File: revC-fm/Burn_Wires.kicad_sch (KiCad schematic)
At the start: 14 parts, among them Q19 MMBT2222AWT3G, Q20 DMN100-7-F, Q21 DMN100-7-F, Q22 IRF7404TRPBF, Q23 IRF7404TRPBF, U23 PE014006

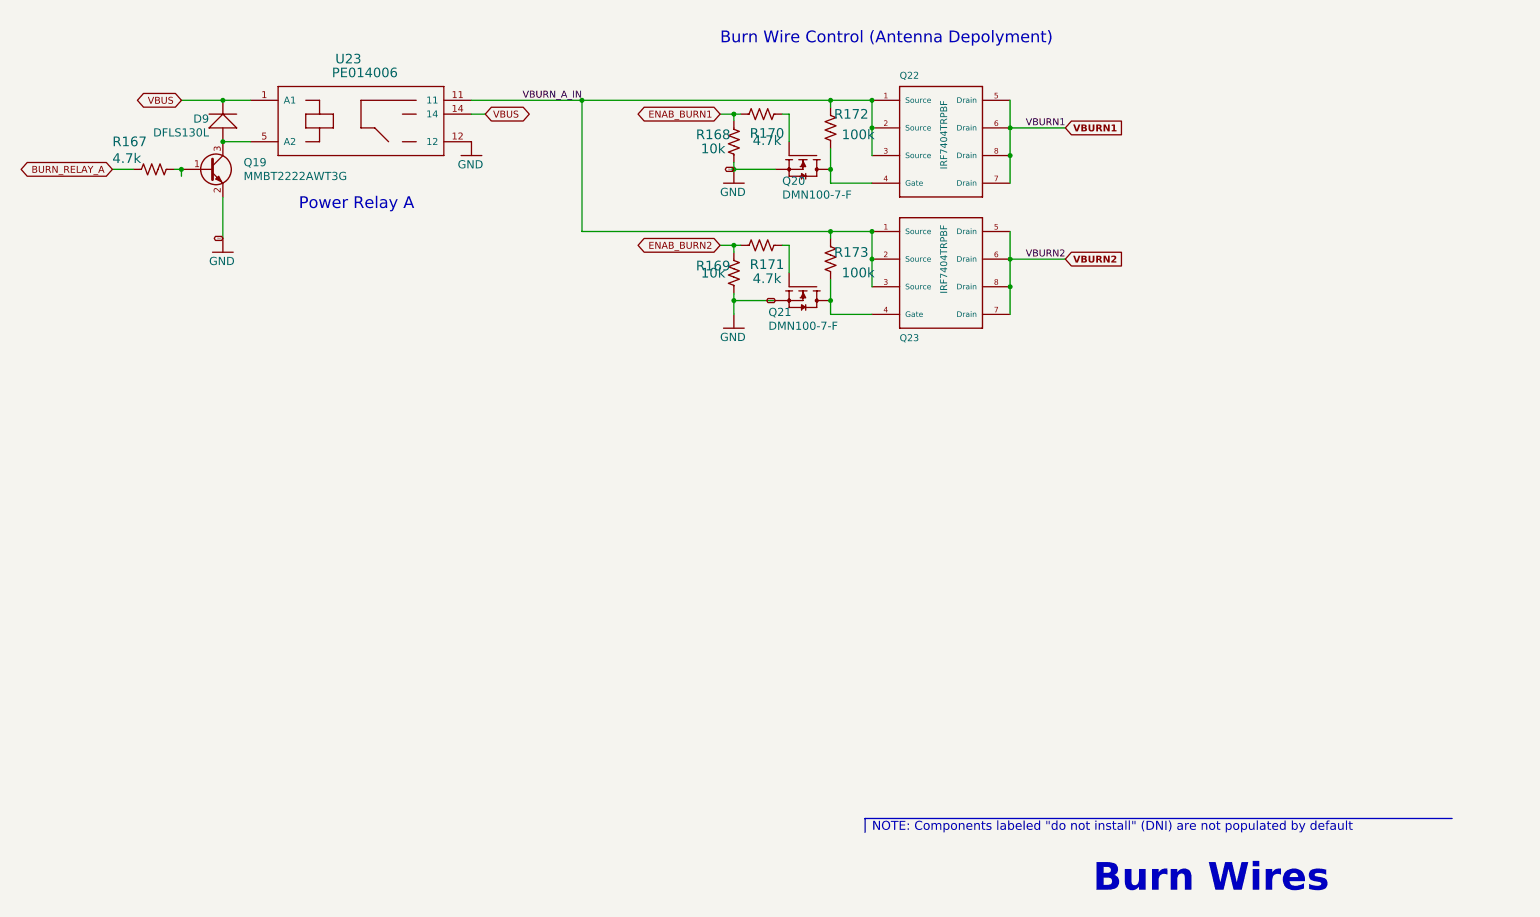
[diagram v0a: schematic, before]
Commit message: working revC
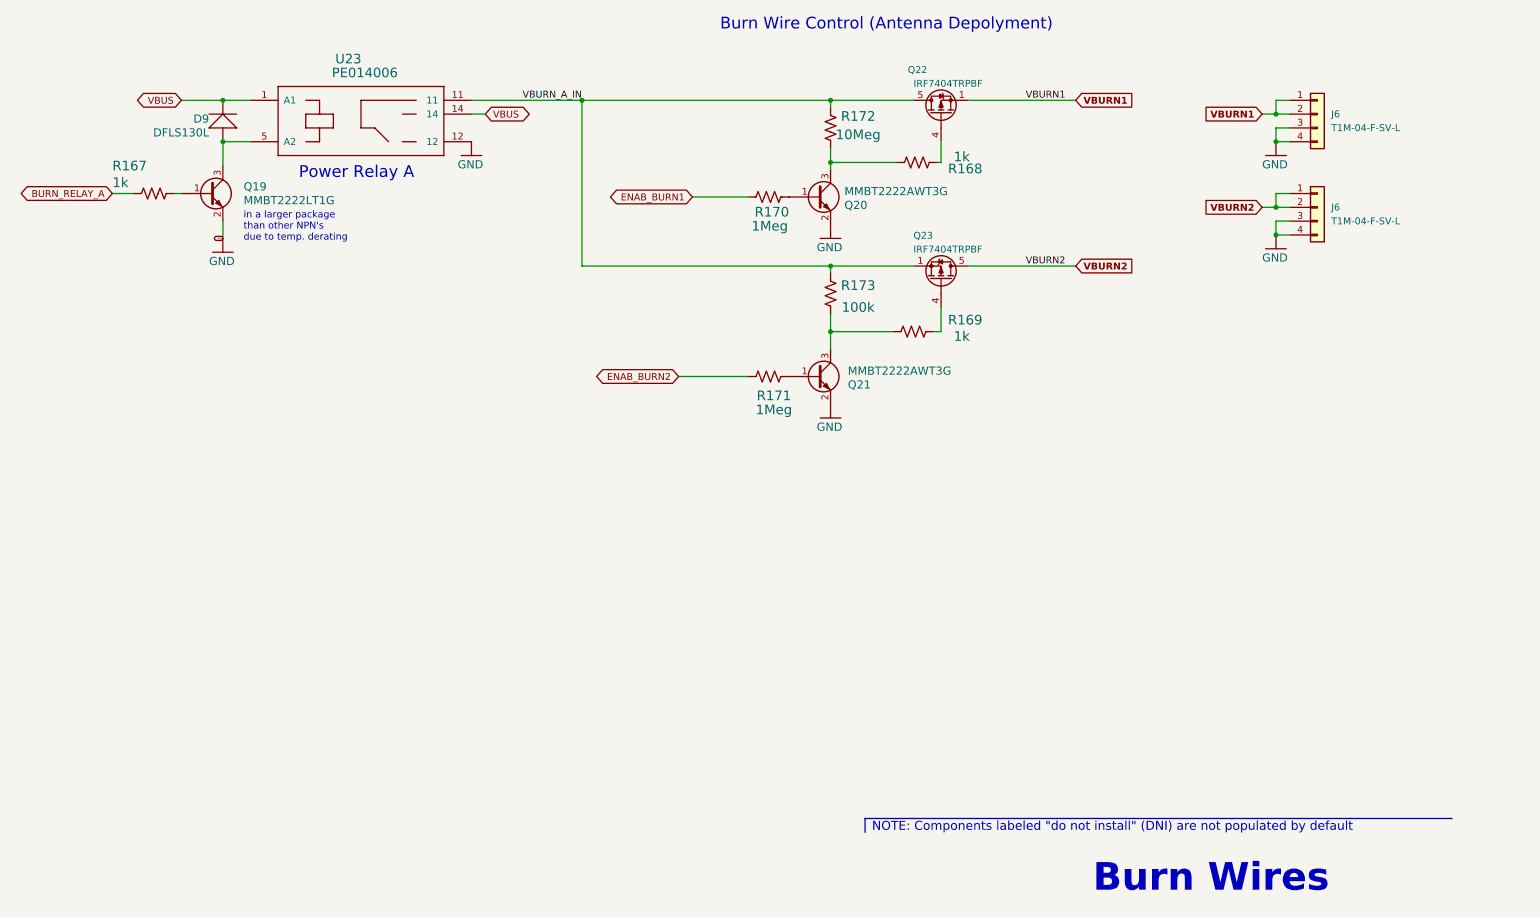
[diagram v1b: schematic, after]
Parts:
- added J6 (x2): T1M-04-F-SV-L, mainboard-SLI:T1M-04-F-SV-L, symbol Connector_Generic:Conn_01x04
- Q19: value MMBT2222AWT3G -> MMBT2222LT1G; footprint Package_TO_SOT_SMD:SOT-323_SC-70 -> Package_TO_SOT_SMD:SOT-23-3
- Q20, Q21: value DMN100-7-F -> MMBT2222AWT3G; footprint mainboard:SOT-23 -> Package_TO_SOT_SMD:SOT-323_SC-70; symbol mainboard:IRLML2803TRPBF -> Device:Q_NPN_BEC; Flight DMN100-7-F -> (none)
- Q22, Q23: symbol mainboard:NDS8434 -> mainboard_SLI:IRF7404TRPBF; Flight IRF7404TRPBF -> (none)
- R167: value 4.7k -> 1k
- R168, R169: value 10k -> 1k
- R170, R171: value 4.7k -> 1Meg
- R172: value 100k -> 10Meg
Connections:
- net ENAB_BURN1: no longer R168.1
- net ENAB_BURN2: no longer R169.1
- net GND: now also J6.3 (Pin_3), J6.3 (Pin_3), J6.4 (Pin_4), J6.4 (Pin_4); no longer R168.2, R169.2
- net VBURN1: now also Q22.1 (S), Q22.2 (S), Q22.3 (S), J6.1 (Pin_1), J6.2 (Pin_2); no longer Q22.5 (Drain), Q22.6 (Drain), Q22.7 (Drain), Q22.8 (Drain)
- net VBURN2: now also J6.1 (Pin_1), J6.2 (Pin_2)
- net VBURN_A_IN: now also Q22.5 (D), Q22.6 (D), Q22.7 (D), Q22.8 (D); no longer Q22.1 (Source), Q22.2 (Source), Q22.3 (Source)
- net at Q20.3 (C), R172.1: now also R168.1; no longer Q22.4 (Gate)
- net at Q21.3 (C), R173.1: now also R169.1; no longer Q23.4 (Gate)
- new net: Q23.4 (G), R169.2
- new net: Q22.4 (G), R168.2
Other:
- note added: "in a larger package than other NPN's due to temp. derating"
- moved on the sheet: Q19, R167, R168, R169, R170, R171, R173

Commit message: working revC
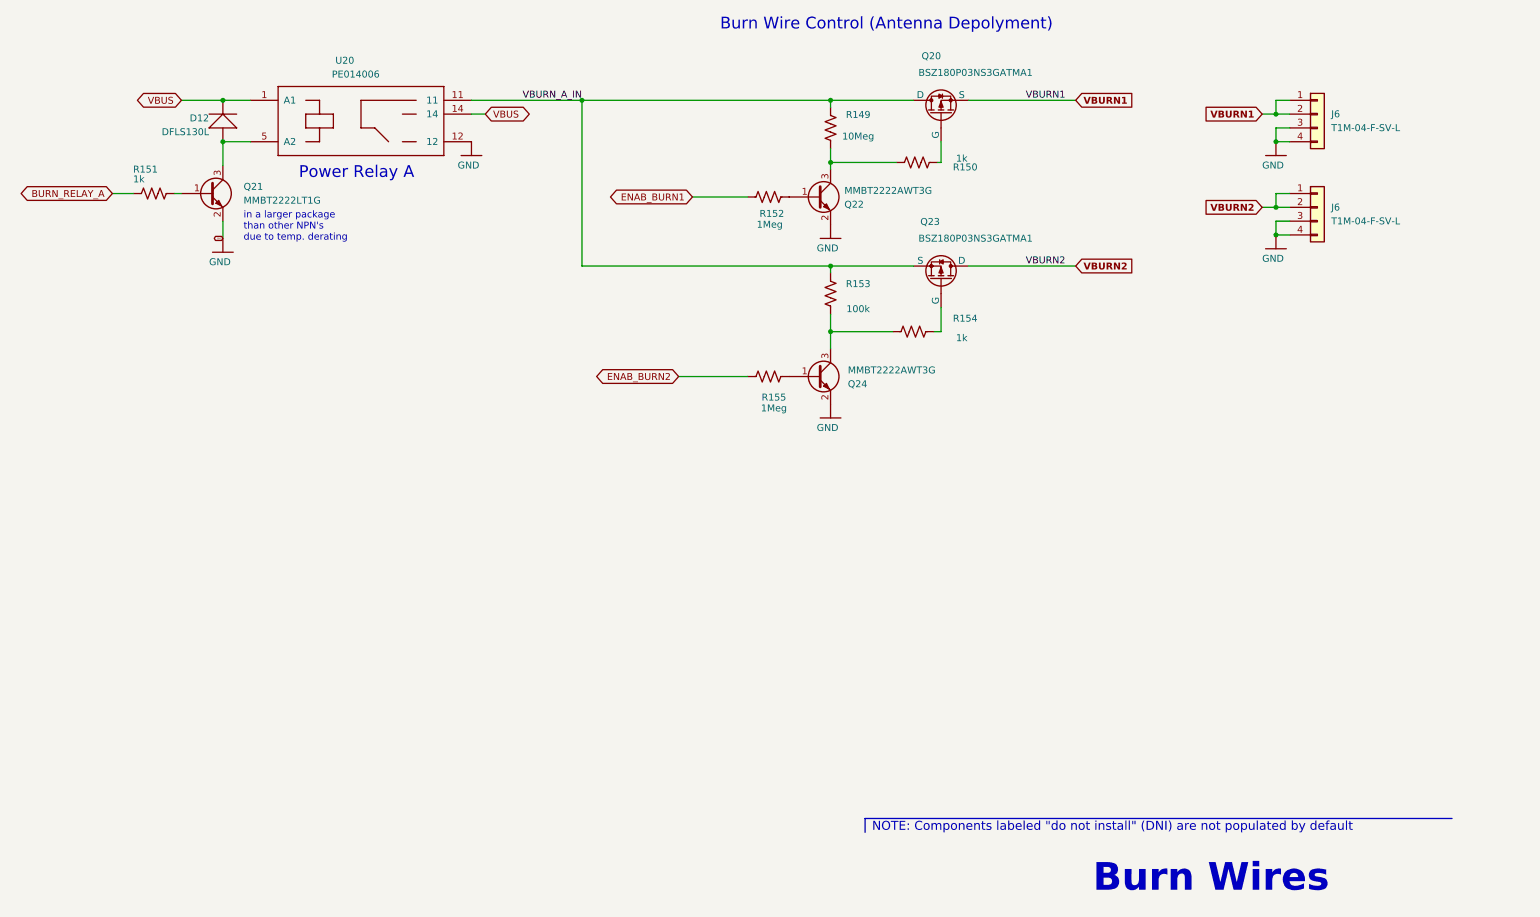
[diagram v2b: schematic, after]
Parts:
- Q20: renamed from Q22; value IRF7404TRPBF -> BSZ180P03NS3GATMA1; footprint Package_SO:SOIC-8_3.9x4.9mm_P1.27mm -> mainboard-SLI:PG-TSDSON-8_3.3x3.3mm; symbol mainboard_SLI:IRF7404TRPBF -> mainboard_SLI:BSZ180
- Q23: value IRF7404TRPBF -> BSZ180P03NS3GATMA1; footprint Package_SO:SOIC-8_3.9x4.9mm_P1.27mm -> mainboard-SLI:PG-TSDSON-8_3.3x3.3mm; symbol mainboard_SLI:IRF7404TRPBF -> mainboard_SLI:BSZ180
- renumbered D9 to D12, Q19 to Q21, Q20 to Q22, Q21 to Q24, R172 to R149, R168 to R150, R167 to R151, R170 to R152, R173 to R153, R169 to R154, R171 to R155, U23 to U20
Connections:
- net VBURN1: no longer Q20.2 (S), Q20.3 (S)
- net VBURN2: no longer Q23.6 (D), Q23.7 (D), Q23.8 (D)
- net VBURN_A_IN: no longer Q20.6 (D), Q20.7 (D), Q20.8 (D), Q23.2 (S), Q23.3 (S)
